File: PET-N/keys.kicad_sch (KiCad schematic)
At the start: 87 parts, among them J1 Extended_PET_keyboard_connect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, SW1 KP "=", SW10 KP "0", SW11 R SHIFT, SW12 ">", SW14 "]", SW15 "@", SW16 L SHIFT, SW17 KP "+", SW18 KP "2", SW2 KP ".", SW20 "?", SW21 ",", SW22 "N", SW23 "V", SW24 "X", SW25 KP "3", SW26 KP "1", SW27 RETURN, SW28 ";", SW29 "M", SW3 NC ($10), SW30 "B", SW31 "C", SW32 "Z", SW320 S LOCK, SW33 KP "*", SW34 KP "5", SW36 ":", SW37 "K", SW38 "H", SW39 "F", SW4 STOP, SW40 "S", SW41 KP "6", SW42 KP "4", SW44 "L", SW45 "J", SW46 "G", SW47 "D", SW48 "A", SW49 KP "/", SW5 "<", SW50 KP "8", SW52 "P", SW53 "I", SW54 "Y", SW55 "R", SW56 "W", SW57 KP "9", SW58 KP "7", SW59 U ARROW, SW6 SPACE, SW60 "O", SW61 "U", SW62 "T", SW63 "E", SW64 "Q", SW65 INS/DEL, SW66 UP/DOWN, SW67 NC ($0A), SW68 ")", SW69 "\", SW7 "[", SW70 "'", SW71 "$", SW72 QUOTE, SW73 LEFT/RIGHT, SW74 CLR/HOME, SW75 B ARROW, SW76 "(", SW77 "&", SW78 "%", SW79 "#", SW8 OFF/RVS, SW80 "!", SW9 KP "-"

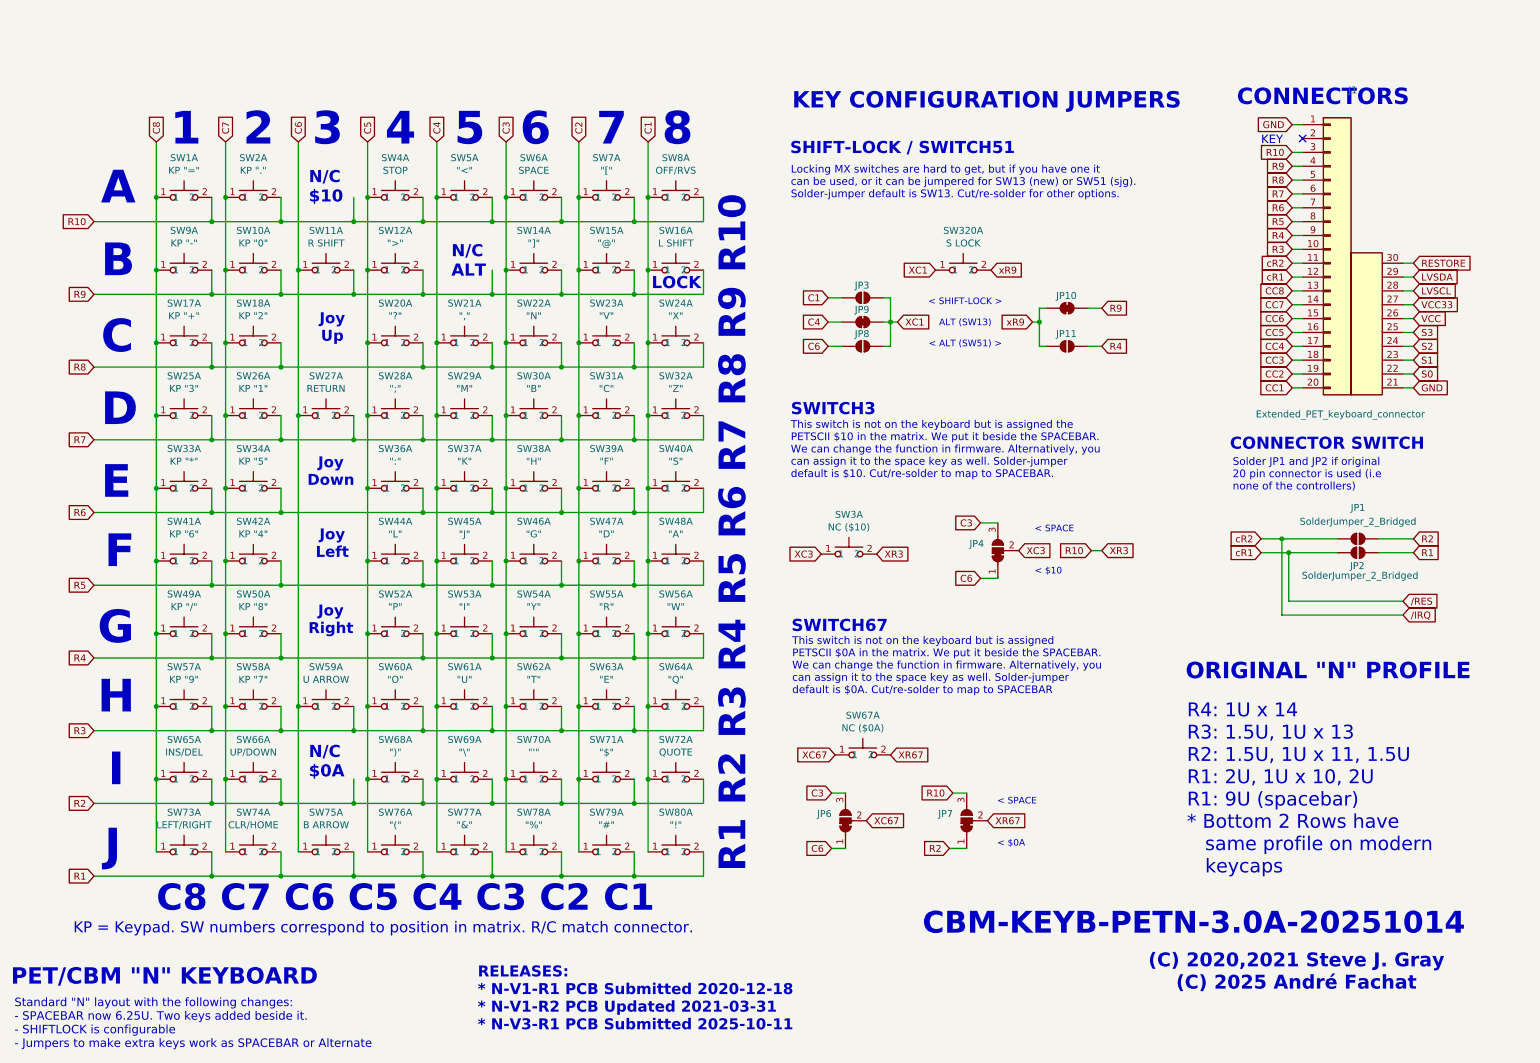
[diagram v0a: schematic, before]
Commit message: first run on r3.1
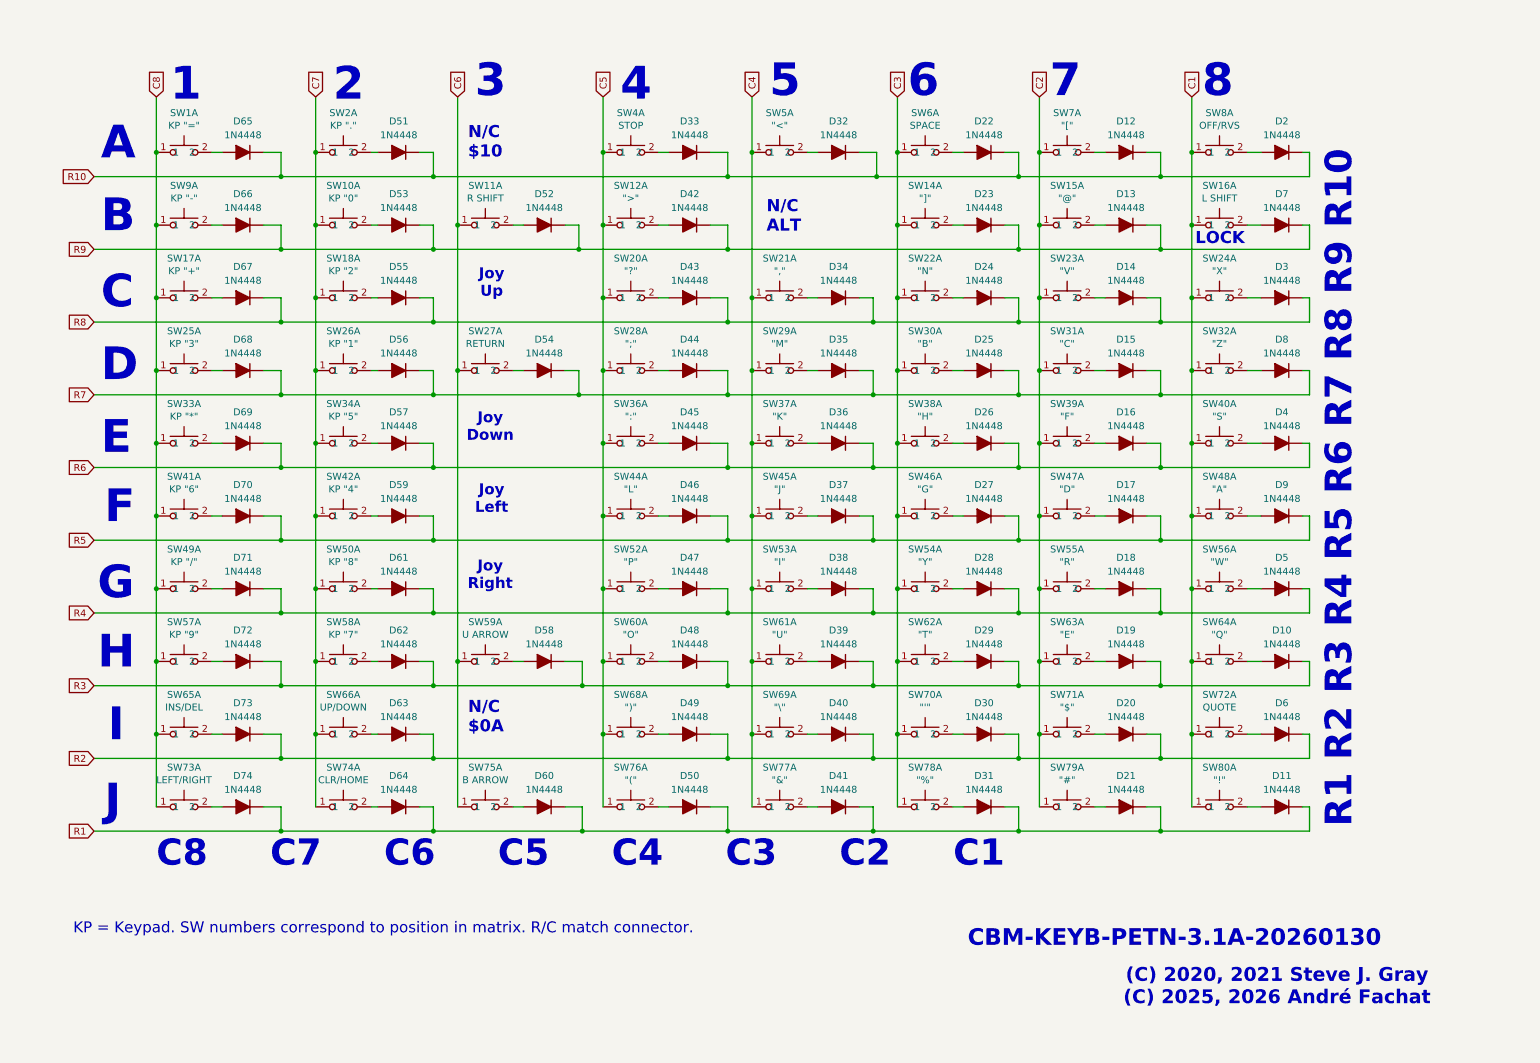
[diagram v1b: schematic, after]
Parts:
- removed J1: Extended_PET_keyboard_connector, petkn:PET_Extended_Keyboard_Connector, symbol petkn:Extended_PET_keyboard_connector
- removed JP1, JP11, JP2, JP3, JP8: SolderJumper_2_Bridged, Jumper:SolderJumper-2_P1.3mm_Open_RoundedPad1.0x1.5mm, symbol Jumper:SolderJumper_2_Open
- removed JP10, JP9: SolderJumper_2_Bridged, Jumper:SolderJumper-2_P1.3mm_Bridged_RoundedPad1.0x1.5mm, symbol Jumper:SolderJumper_2_Bridged
- removed JP4, JP6, JP7: SolderJumper_3_Bridged12, Jumper:SolderJumper-3_P1.3mm_Bridged12_RoundedPad1.0x1.5mm_NumberLabels, symbol Jumper:SolderJumper_3_Bridged12
- removed SW3: NC ($10), petkn:SW_Cherry_MX_1.25u_PCB_with_RGB_LED, symbol petkn:MX Key with SMD RGB LED
- removed SW320: S LOCK, petkn:SW_Cherry_MX_1.50u_PCB_with_RGB_LED, symbol petkn:MX Key with SMD RGB LED
- removed SW67: NC ($0A), petkn:SW_Cherry_MX_1.50u_PCB_with_RGB_LED, symbol petkn:MX Key with SMD RGB LED
- added D10, D11, D12, D13, D14, D15, D16, D17, D18, D19, D2, D20, D21, D22, D23, D24, D25, D26, D27, D28, D29, D3, D30, D31, D32, D33, D34, D35, D36, D37, D38, D39, D4, D40, D41, D42, D43, D44, D45, D46, D47, D48, D49, D5, D50, D51, D52, D53, D54, D55, D56, D57, D58, D59, D6, D60, D61, D62, D63, D64, D65, D66, D67, D68, D69, D7, D70, D71, D72, D73, D74, D8, D9: 1N4448, Diode_SMD:D_SOD-323_HandSoldering, symbol PCM_Diode_AKL:1N4448
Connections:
- net R1: now also D11.1 (K), D21.1 (K), D31.1 (K), D41.1 (K), D50.1 (K), D60.1 (K), D64.1 (K), D74.1 (K); no longer SW73.2, SW74.2, SW75.2, SW76.2, SW77.2, SW78.2, SW79.2, SW80.2
- net R10: now also D12.1 (K), D2.1 (K), D22.1 (K), D32.1 (K), D33.1 (K), D51.1 (K), D65.1 (K); no longer SW1.2, SW2.2, SW4.2, SW5.2, SW6.2, SW7.2, SW8.2
- net R2: now also D20.1 (K), D30.1 (K), D40.1 (K), D49.1 (K), D6.1 (K), D63.1 (K), D73.1 (K); no longer SW65.2, SW66.2, SW68.2, SW69.2, SW70.2, SW71.2, SW72.2
- net R3: now also D10.1 (K), D19.1 (K), D29.1 (K), D39.1 (K), D48.1 (K), D58.1 (K), D62.1 (K), D72.1 (K); no longer SW57.2, SW58.2, SW59.2, SW60.2, SW61.2, SW62.2, SW63.2, SW64.2
- net R4: now also D18.1 (K), D28.1 (K), D38.1 (K), D47.1 (K), D5.1 (K), D61.1 (K), D71.1 (K); no longer SW49.2, SW50.2, SW52.2, SW53.2, SW54.2, SW55.2, SW56.2
- net R5: now also D17.1 (K), D27.1 (K), D37.1 (K), D46.1 (K), D59.1 (K), D70.1 (K), D9.1 (K); no longer SW41.2, SW42.2, SW44.2, SW45.2, SW46.2, SW47.2, SW48.2
- net R6: now also D16.1 (K), D26.1 (K), D36.1 (K), D4.1 (K), D45.1 (K), D57.1 (K), D69.1 (K); no longer SW33.2, SW34.2, SW36.2, SW37.2, SW38.2, SW39.2, SW40.2
- net R7: now also D15.1 (K), D25.1 (K), D35.1 (K), D44.1 (K), D54.1 (K), D56.1 (K), D68.1 (K), D8.1 (K); no longer SW25.2, SW26.2, SW27.2, SW28.2, SW29.2, SW30.2, SW31.2, SW32.2
- net R8: now also D14.1 (K), D24.1 (K), D3.1 (K), D34.1 (K), D43.1 (K), D55.1 (K), D67.1 (K); no longer SW17.2, SW18.2, SW20.2, SW21.2, SW22.2, SW23.2, SW24.2
- net R9: now also D13.1 (K), D23.1 (K), D42.1 (K), D52.1 (K), D53.1 (K), D66.1 (K), D7.1 (K); no longer SW10.2, SW11.2, SW12.2, SW14.2, SW15.2, SW16.2, SW9.2
- new net: D65.2 (A), SW1.2
- new net: D51.2 (A), SW2.2
- new net: D33.2 (A), SW4.2
- new net: D32.2 (A), SW5.2
- new net: D22.2 (A), SW6.2
- new net: D12.2 (A), SW7.2
- new net: D2.2 (A), SW8.2
- new net: D66.2 (A), SW9.2
- new net: D53.2 (A), SW10.2
- new net: D52.2 (A), SW11.2
- new net: D42.2 (A), SW12.2
- new net: D23.2 (A), SW14.2
- new net: D13.2 (A), SW15.2
- new net: D7.2 (A), SW16.2
- new net: D67.2 (A), SW17.2
- new net: D55.2 (A), SW18.2
- new net: D43.2 (A), SW20.2
- new net: D34.2 (A), SW21.2
- new net: D24.2 (A), SW22.2
- new net: D14.2 (A), SW23.2
- new net: D3.2 (A), SW24.2
- new net: D68.2 (A), SW25.2
- new net: D56.2 (A), SW26.2
- new net: D54.2 (A), SW27.2
- new net: D44.2 (A), SW28.2
- new net: D35.2 (A), SW29.2
- new net: D25.2 (A), SW30.2
- new net: D15.2 (A), SW31.2
- new net: D8.2 (A), SW32.2
- new net: D69.2 (A), SW33.2
- new net: D57.2 (A), SW34.2
- new net: D45.2 (A), SW36.2
- new net: D36.2 (A), SW37.2
- new net: D26.2 (A), SW38.2
- new net: D16.2 (A), SW39.2
- new net: D4.2 (A), SW40.2
- new net: D70.2 (A), SW41.2
- new net: D59.2 (A), SW42.2
- new net: D46.2 (A), SW44.2
- new net: D37.2 (A), SW45.2
- new net: D27.2 (A), SW46.2
- new net: D17.2 (A), SW47.2
- new net: D9.2 (A), SW48.2
- new net: D71.2 (A), SW49.2
- new net: D61.2 (A), SW50.2
- new net: D47.2 (A), SW52.2
- new net: D38.2 (A), SW53.2
- new net: D28.2 (A), SW54.2
- new net: D18.2 (A), SW55.2
- new net: D5.2 (A), SW56.2
- new net: D72.2 (A), SW57.2
- new net: D62.2 (A), SW58.2
- new net: D58.2 (A), SW59.2
- new net: D48.2 (A), SW60.2
- new net: D39.2 (A), SW61.2
- new net: D29.2 (A), SW62.2
- new net: D19.2 (A), SW63.2
- new net: D10.2 (A), SW64.2
- new net: D73.2 (A), SW65.2
- new net: D63.2 (A), SW66.2
- new net: D49.2 (A), SW68.2
- new net: D40.2 (A), SW69.2
- new net: D30.2 (A), SW70.2
- new net: D20.2 (A), SW71.2
- new net: D6.2 (A), SW72.2
- new net: D74.2 (A), SW73.2
- new net: D64.2 (A), SW74.2
- new net: D60.2 (A), SW75.2
- new net: D50.2 (A), SW76.2
- new net: D41.2 (A), SW77.2
- new net: D31.2 (A), SW78.2
- new net: D21.2 (A), SW79.2
- new net: D11.2 (A), SW80.2
- no-connect marks 1 -> 0
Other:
- note added: "(C) 2020, 2021 Steve J. Gray (C) 2025, 2026 André Fachat"
- note added: "CBM-KEYB-PETN-3.1A-20260130"
- note removed: "(C) 2020,2021 Steve J. Gray (C) 2025 André Fachat"
- note removed: "< SHIFT-LOCK > ALT (SW13) < ALT (SW51) >"
- note removed: "< SPACE < $0A"
- note removed: "< SPACE < $10"
- note removed: "CBM-KEYB-PETN-3.0A-20251014"
- note removed: "CONNECTOR SWITCH"
- note removed: "CONNECTORS"
- note removed: "KEY"
- note removed: "KEY CONFIGURATION JUMPERS"
- note removed: "Locking MX switches are hard to get, but if you have one it can be used, or it can be jumpered for SW13 (new) or SW51 (sjg). Solder-jumper default is SW13. Cut/re-solder for other options."
- note removed: "ORIGINAL "N" PROFILE"
- note removed: "PET/CBM "N" KEYBOARD"
- note removed: "R4: 1U x 14 R3: 1.5U, 1U x 13 R2: 1.5U, 1U x 11, 1.5U R1: 2U, 1U x 10, 2U R1: 9U (spacebar) * Bottom 2 Rows have same profile on modern keycaps"
- note removed: "RELEASES: * N-V1-R1 PCB Submitted 2020-12-18 * N-V1-R2 PCB Updated 2021-03-31 * N-V3-R1 PCB Submitted 2025-10-11"
- note removed: "SHIFT-LOCK / SWITCH51"
- note removed: "SWITCH3"
- note removed: "SWITCH67"
- note removed: "Solder JP1 and JP2 if original 20 pin connector is used (i.e none of the controllers)"
- note removed: "Standard "N" layout with the following changes: - SPACEBAR now 6.25U. Two keys added beside it. - SHIFTLOCK is configurable - Jumpers to make extra keys work as SPACEBAR or Alternate"
- note removed: "This switch is not on the keyboard but is assigned PETSCII $0A in the matrix. We put it beside the SPACEBAR. We can change the function in firmware. Alternatively, you can assign it to the space key as well. Solder-jumper default is $0A. Cut/re-solder to map to SPACEBAR"
- note removed: "This switch is not on the keyboard but is assigned the PETSCII $10 in the matrix. We put it beside the SPACEBAR. We can change the function in firmware. Alternatively, you can assign it to the space key as well. Solder-jumper default is $10. Cut/re-solder to map to SPACEBAR."
- moved on the sheet: SW10A, SW11A, SW12A, SW14A, SW15A, SW16A, SW17A, SW18A, SW1A, SW20A, SW21A, SW22A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
